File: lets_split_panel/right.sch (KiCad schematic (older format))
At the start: 69 parts, among them J4 RST, J5 Speaker, J6 ISP, P5 USB_OTG, P6 >WS2812, P7 WS2812>, P8 Conn_01x04, SW25 MXALPS, SW26 MXALPS, SW27 MXALPS, SW28 MXALPS, SW29 MXALPS, SW30 MXALPS, SW31 MXALPS, SW32 MXALPS, SW33 MXALPS, SW34 MXALPS, SW35 MXALPS, SW36 MXALPS, SW37 MXALPS, SW38 MXALPS, SW39 MXALPS, SW40 MXALPS, SW41 MXALPS, SW42 MXALPS, SW43 MXALPS, SW44 MXALPS, SW45 MXALPS, SW46 MXALPS, SW47 MXALPS, SW48 MXALPS, U2 ATMega32U4, Y2 Crystal

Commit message: Finished panel
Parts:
- removed JP3, JP4: I2C pullup, Jumpers:Solder-jumper-NO, symbol Jumper
- removed R11, R12: 4k7, Resistors_SMD:R_0603_HandSoldering, symbol R_Small
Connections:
- net labels added: Dd+, Dd-
- wire segments 132 -> 124
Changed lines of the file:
@@
 	1    0    0    -1
 $EndComp
-Text GLabel 4225 6625 2    55   Input ~ 0
+Text Label 4225 6625 0    55   ~ 0
 col0
-Text GLabel 4225 6725 2    55   Input ~ 0
+Text Label 4225 6725 0    55   ~ 0
 col1
-Text GLabel 4225 6275 2    55   Input ~ 0
+Text Label 4225 6275 0    55   ~ 0
 col2
-Text GLabel 4225 4925 2    55   Input ~ 0
+Text Label 4225 4925 0    55   ~ 0
 col3
-Text GLabel 4225 6125 2    55   Input ~ 0
+Text Label 4225 6125 0    55   ~ 0
 col4
-Text GLabel 4225 6025 2    55   Input ~ 0
+Text Label 4225 6025 0    55   ~ 0
 col5
-Text GLabel 4225 7025 2    55   Input ~ 0
+Text Label 4225 7025 0    55   ~ 0
 row3
-Text GLabel 4225 5275 2    55   Input ~ 0
+Text Label 4225 5275 0    55   ~ 0
 row2
-Text GLabel 4225 6925 2    55   Input ~ 0
+Text Label 4225 6925 0    55   ~ 0
 row1
-Text GLabel 4225 6825 2    55   Input ~ 0
+Text Label 4225 6825 0    55   ~ 0
 row0
 $Comp
@@
 	1    0    0    -1
 $EndComp
-$Comp
-L R_Small R12
-U 1 1 5A0E2942
-P 3525 1750
-F 0 "R12" H 3555 1770 50  0000 L CNN
-F 1 "4k7" H 3555 1710 50  0000 L CNN
-F 2 "Resistors_SMD:R_0603_HandSoldering" H 3525 1750 50  0001 C CNN
-F 3 "" H 3525 1750 50  0000 C CNN
-	1    3525 1750
-	1    0    0    -1
-$EndComp
-$Comp
-L R_Small R11
-U 1 1 5A0E2948
-P 3425 1750
-F 0 "R11" H 3455 1770 50  0000 L CNN
-F 1 "4k7" H 3455 1710 50  0000 L CNN
-F 2 "Resistors_SMD:R_0603_HandSoldering" H 3425 1750 50  0001 C CNN
-F 3 "" H 3425 1750 50  0000 C CNN
-	1    3425 1750
-	-1   0    0    -1
-$EndComp
-$Comp
-L Jumper JP3
-U 1 1 5A0E294E
-P 3425 1300
-F 0 "JP3" H 3425 1450 50  0000 C CNN
-F 1 "I2C pullup" H 3425 1525 50  0000 C CNN
-F 2 "Jumpers:Solder-jumper-NO" H 3425 1300 50  0001 C CNN
-F 3 "" H 3425 1300 50  0000 C CNN
-	1    3425 1300
-	0    -1   1    0
-$EndComp
-$Comp
-L VCC #PWR024
-U 1 1 5A0E2954
-P 3475 925
-F 0 "#PWR024" H 3475 775 50  0001 C CNN
-F 1 "VCC" H 3475 1075 50  0000 C CNN
-F 2 "" H 3475 925 50  0000 C CNN
-F 3 "" H 3475 925 50  0000 C CNN
-	1    3475 925
-	1    0    0    -1
-$EndComp
-Text GLabel 3675 1900 2    55   Output ~ 0
-SDA
-Text GLabel 3675 2000 2    55   Output ~ 0
+Text Label 7400 2900 2    55   ~ 0
 SCL/D3
-Text GLabel 7400 2900 0    55   Input ~ 0
-SCL/D3
-Text GLabel 7400 2800 0    55   Input ~ 0
+Text Label 7400 2800 2    55   ~ 0
 SDA
 $Comp
 L USB_OTG-RESCUE-lets_split P5
 U 1 1 5A0E295E
-P 1225 5525
-F 0 "P5" H 1550 5400 50  0000 C CNN
-F 1 "USB_OTG" H 1225 5725 50  0000 C CNN
-F 2 "Connectors:USB-Mini-B-SMD" V 1175 5425 50  0001 C CNN
-F 3 "" V 1175 5425 50  0000 C CNN
-	1    1225 5525
+P 1150 5525
+F 0 "P5" H 1475 5400 50  0000 C CNN
+F 1 "USB_OTG" H 1150 5725 50  0000 C CNN
+F 2 "Connectors:USB-Mini-B-SMD" V 1100 5425 50  0001 C CNN
+F 3 "" V 1100 5425 50  0000 C CNN
+	1    1150 5525
 	0    -1   1    0
 $EndComp
@@
 	1    0    0    -1
 $EndComp
-Text GLabel 4250 6525 2    55   Output ~ 0
+Text Label 4250 6525 0    55   ~ 0
 WD2812-in
-Text GLabel 3075 2525 0    55   Input ~ 0
+Text Label 3075 2525 2    55   ~ 0
 WD2812-in
 $Comp
@@
 	-1   0    0    -1
 $EndComp
-Text GLabel 3900 2525 2    55   Output ~ 0
+Text Label 3900 2525 0    55   ~ 0
 SDA
-Text GLabel 3275 1900 0    55   Input ~ 0
+Text Label 4275 5525 0    55   ~ 0
 SDA
-Text GLabel 3275 2000 0    55   Input ~ 0
+Text Label 4275 5425 0    55   ~ 0
 SCL/D3
-Text GLabel 4275 5525 2    55   Output ~ 0
-SDA
-Text GLabel 4275 5425 2    55   Output ~ 0
-SCL/D3
-Text GLabel 4275 5175 2    60   Output ~ 0
+Text Label 4275 5175 0    60   ~ 0
 buzz
-Text GLabel 3200 3125 0    60   Input ~ 0
+Text Label 3200 3125 2    60   ~ 0
 buzz
 $Comp
@@
 L VBUS #PWR031
 U 1 1 5A0E29DF
-P 1575 5275
-F 0 "#PWR031" H 1575 5125 50  0001 C CNN
-F 1 "VBUS" H 1590 5448 50  0000 C CNN
-F 2 "" H 1575 5275 50  0001 C CNN
-F 3 "" H 1575 5275 50  0001 C CNN
-	1    1575 5275
+P 1500 5275
+F 0 "#PWR031" H 1500 5125 50  0001 C CNN
+F 1 "VBUS" H 1515 5448 50  0000 C CNN
+F 2 "" H 1500 5275 50  0001 C CNN
+F 3 "" H 1500 5275 50  0001 C CNN
+	1    1500 5275
 	1    0    0    -1
 $EndComp
@@
 L GND #PWR033
 U 1 1 5A0E29EB
-P 1125 6050
-F 0 "#PWR033" H 1125 5800 50  0001 C CNN
-F 1 "GND" H 1125 5900 50  0000 C CNN
-F 2 "" H 1125 6050 50  0000 C CNN
-F 3 "" H 1125 6050 50  0000 C CNN
-	1    1125 6050
+P 1050 6050
+F 0 "#PWR033" H 1050 5800 50  0001 C CNN
+F 1 "GND" H 1050 5900 50  0000 C CNN
+F 2 "" H 1050 6050 50  0000 C CNN
+F 3 "" H 1050 6050 50  0000 C CNN
+	1    1050 6050
 	1    0    0    -1
 $EndComp
@@
 	2350 4200 2350 5225
 Wire Wire Line
-	3275 2000 3675 2000
-Wire Wire Line
-	3525 2000 3525 1850
-Wire Wire Line
-	3275 1900 3675 1900
-Wire Wire Line
-	3425 1900 3425 1850
-Wire Wire Line
-	3425 1650 3425 1600
-Wire Wire Line
-	3525 1600 3525 1650
-Connection ~ 3425 1900
-Connection ~ 3525 2000
-Wire Wire Line
 	7350 3150 7350 3100
 Wire Wire Line
@@
 	2625 5525 1725 5525
 Wire Wire Line
-	1525 5325 1575 5325
-Wire Wire Line
-	1575 5325 1575 5275
-Wire Wire Line
-	1125 5925 1125 6050
+	1450 5325 1500 5325
+Wire Wire Line
+	1500 5325 1500 5275
+Wire Wire Line
+	1050 5925 1050 6050
 Wire Wire Line
 	2100 5725 2275 5725
@@
 	2100 5725 2100 6200
 Wire Wire Line
-	1125 5975 1575 5975
-Wire Wire Line
-	1575 5975 1575 5725
-Wire Wire Line
-	1575 5725 1525 5725
-Connection ~ 1125 5975
+	1050 5975 1500 5975
+Wire Wire Line
+	1500 5975 1500 5725
+Wire Wire Line
+	1500 5725 1450 5725
+Connection ~ 1050 5975
 $Comp
 L VBUS #PWR034
@@
 	4225 6525 4250 6525
 $Comp
-L Jumper JP4
-U 1 1 5A0E2A65
-P 3525 1300
-F 0 "JP4" H 3525 1450 50  0000 C CNN
-F 1 "I2C pullup" H 3525 1525 50  0000 C CNN
-F 2 "Jumpers:Solder-jumper-NO" H 3525 1300 50  0001 C CNN
-F 3 "" H 3525 1300 50  0000 C CNN
-	1    3525 1300
-	0    1    1    0
-$EndComp
-Wire Wire Line
-	3425 1000 3425 975
-Wire Wire Line
-	3425 975  3525 975
-Wire Wire Line
-	3525 975  3525 1000
-Wire Wire Line
-	3475 975  3475 925
-Connection ~ 3475 975
-$Comp
 L Conn_02x03_Odd_Even J6
 U 1 1 5A0E2A70
@@
 	1    0    0    -1
 $EndComp
-Text GLabel 5575 6800 0    35   Output ~ 0
+Text Label 5575 6800 2    55   ~ 0
 ~RESET
-Text GLabel 5575 6600 0    55   Input ~ 0
-MISO
-Text GLabel 5575 6700 0    55   Output ~ 0
+Text Label 5575 6700 2    55   ~ 0
 SCK
-Text GLabel 6075 6700 2    55   Output ~ 0
-MOSI
-Text GLabel 1925 4725 1    35   Input ~ 0
+Text Label 1925 4725 1    35   ~ 0
 ~RESET
 Wire Wire Line
 	1925 4725 1925 4775
 Connection ~ 1925 4775
-Text GLabel 4225 4525 2    55   Input ~ 0
+Text Label 4225 4525 0    55   ~ 0
 MOSI
-Text GLabel 4225 4625 2    55   Output ~ 0
+Text Label 4225 4625 0    55   ~ 0
 MISO
-Text GLabel 4225 4425 2    55   Input ~ 0
+Text Label 4225 4425 0    55   ~ 0
 SCK
 Wire Wire Line
@@
 $EndComp
 Wire Wire Line
-	10000 4825 9875 4825
+	9875 4825 10000 4825
 Wire Wire Line
 	10400 4825 10475 4825
@@
 $EndComp
 Wire Wire Line
-	9250 4825 9125 4825
+	9125 4825 9250 4825
 Wire Wire Line
 	9650 4825 9725 4825
@@
 $EndComp
 Wire Wire Line
-	8500 4825 8375 4825
+	8375 4825 8500 4825
 Wire Wire Line
 	8900 4825 8975 4825
@@
 $EndComp
 Wire Wire Line
-	7750 4825 7625 4825
+	7625 4825 7750 4825
 Wire Wire Line
 	8150 4825 8225 4825
@@
 $EndComp
 Wire Wire Line
-	7050 4825 6925 4825
+	6925 4825 7050 4825
 Wire Wire Line
 	7450 4825 7525 4825
@@
 $EndComp
 Wire Wire Line
-	6300 4825 6175 4825
+	6175 4825 6300 4825
 Wire Wire Line
 	6700 4825 6775 4825
@@
 $EndComp
 Wire Wire Line
-	10000 4325 9875 4325
+	9875 4325 10000 4325
 Wire Wire Line
 	10400 4325 10475 4325
@@
 $EndComp
 Wire Wire Line
-	9250 4325 9125 4325
+	9125 4325 9250 4325
 Wire Wire Line
 	9650 4325 9725 4325
@@
 $EndComp
 Wire Wire Line
-	8500 4325 8375 4325
+	8375 4325 8500 4325
 Wire Wire Line
 	8900 4325 8975 4325
@@
 $EndComp
 Wire Wire Line
-	7750 4325 7625 4325
+	7625 4325 7750 4325
 Wire Wire Line
 	8150 4325 8225 4325
@@
 $EndComp
 Wire Wire Line
-	7050 4325 6925 4325
+	6925 4325 7050 4325
 Wire Wire Line
 	7450 4325 7525 4325
@@
 $EndComp
 Wire Wire Line
-	6300 4325 6175 4325
+	6175 4325 6300 4325
 Wire Wire Line
 	6700 4325 6775 4325
@@
 Wire Wire Line
 	6775 4125 10475 4125
-Text GLabel 6775 5625 0    60   Input ~ 0
+Text Label 6775 5625 2    60   ~ 0
 row3
-Text GLabel 6775 5125 0    60   Input ~ 0
+Text Label 6775 5125 2    60   ~ 0
 row2
-Text GLabel 6775 4625 0    60   Input ~ 0
+Text Label 6775 4625 2    60   ~ 0
 row1
-Text GLabel 6775 4125 0    60   Input ~ 0
+Text Label 6775 4125 2    60   ~ 0
 row0
-Text GLabel 9875 3775 1    60   Input ~ 0
+Text Label 9875 3775 1    60   ~ 0
 col5
-Text GLabel 9125 3775 1    60   Input ~ 0
+Text Label 9125 3775 1    60   ~ 0
 col4
-Text GLabel 8375 3775 1    60   Input ~ 0
+Text Label 8375 3775 1    60   ~ 0
 col3
-Text GLabel 7625 3775 1    60   Input ~ 0
+Text Label 7625 3775 1    60   ~ 0
 col2
-Text GLabel 6925 3775 1    60   Input ~ 0
+Text Label 6925 3775 1    60   ~ 0
 col1
-Text GLabel 6175 3775 1    60   Input ~ 0
+Text Label 6175 3775 1    60   ~ 0
 col0
 $Comp
@@
 	0    -1   -1   0
 $EndComp
+Text Label 5575 6600 2    55   ~ 0
+MISO
+Text Label 6075 6700 0    55   ~ 0
+MOSI
+Text Label 1450 5425 0    60   ~ 0
+Dd-
+Wire Wire Line
+	1450 5425 1525 5425
+Text Label 1450 5525 0    60   ~ 0
+Dd+
+Wire Wire Line
+	1450 5525 1525 5525
 $EndSCHEMATC

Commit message: Added test jig for panel
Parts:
- removed P7: WS2812>, Wirepads:SMD_PAD_1x03_Pitch2.54mm, symbol Conn_01x03
- added J8: WS2812>, Pin_Headers:Pin_Header_Straight_1x01_Pitch2.54mm, symbol conn:Conn_01x01
- C5, C6, C7, C8: symbol C_Small -> lets_split_panel-rescue:C_Small-RESCUE-lets_split_panel
- D25, D26, D27, D28, D29, D30, D31, D32, D33, D34, D35, D36, D37, D38, D39, D40, D41, D42, D43, D44, D45, D46, D47, D48: symbol D -> lets_split_panel-rescue:D-RESCUE-lets_split_panel
- J4, J5: symbol Conn_01x02 -> lets_split_panel-rescue:Conn_01x02-RESCUE-lets_split_panel
- J6: footprint Jlink:J-link-needle-6pin -> Pin_Headers:Pin_Header_Straight_2x03_Pitch2.54mm; symbol Conn_02x03_Odd_Even -> lets_split_panel-rescue:Conn_02x03_Odd_Even-RESCUE-lets_split_panel
- P5: symbol USB_OTG-RESCUE-lets_split -> lets_split_panel-rescue:USB_OTG-RESCUE-lets_split-RESCUE-lets_split_panel
- P6: symbol Conn_01x03 -> lets_split_panel-rescue:Conn_01x03-RESCUE-lets_split_panel
- P8: symbol Conn_01x04 -> lets_split_panel-rescue:Conn_01x04-RESCUE-lets_split_panel
- R10, R7, R8, R9: symbol R_Small -> lets_split_panel-rescue:R_Small-RESCUE-lets_split_panel
- SW25, SW26, SW27, SW28, SW29, SW30, SW31, SW32, SW33, SW34, SW35, SW36, SW37, SW38, SW39, SW40, SW41, SW42, SW43, SW44, SW45, SW46, SW47, SW48: symbol MXALPS -> lets_split_panel-rescue:MXALPS-RESCUE-lets_split_panel
- U2: symbol ATMega32U4 -> lets_split_panel-rescue:ATMega32U4-RESCUE-lets_split_panel
- Y2: symbol Crystal -> lets_split_panel-rescue:Crystal-RESCUE-lets_split_panel
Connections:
- wire segments 124 -> 120

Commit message: Changed to use SOT-23 dual diodes for cost
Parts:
- removed D25, D26, D27, D28, D29, D30, D31, D32, D33, D34, D35, D36, D37, D38, D39, D40, D41, D42, D43, D44, D45, D46, D47, D48: D, SeeedOPL-Diode-2016:SOD-123, symbol lets_split_panel-rescue:D-RESCUE-lets_split_panel
- removed SW25, SW26, SW27, SW28, SW29, SW30, SW31, SW32, SW33, SW34, SW35, SW36, SW37, SW38, SW39, SW40, SW41, SW42, SW43, SW44, SW45, SW46, SW47, SW48: MXALPS, CherryMX:Kailh-socket, symbol lets_split_panel-rescue:MXALPS-RESCUE-lets_split_panel
- added D13, D14, D15, D16, D17, D18, D19, D20, D21, D22, D23, D24: D_x2_KCom_AAK, TO_SOT_Packages_SMD:SOT-23, symbol device:D_x2_KCom_AAK
- added SW25, SW26, SW27, SW28, SW29, SW30, SW31, SW32, SW33, SW34, SW35, SW36, SW37, SW38, SW39, SW40, SW41, SW42, SW43, SW44, SW45, SW46, SW47, SW48: Socket, CherryMX:Kailh-socket, symbol switches:SW_Push
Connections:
- wire segments 120 -> 108
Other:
- moved on the sheet: P8

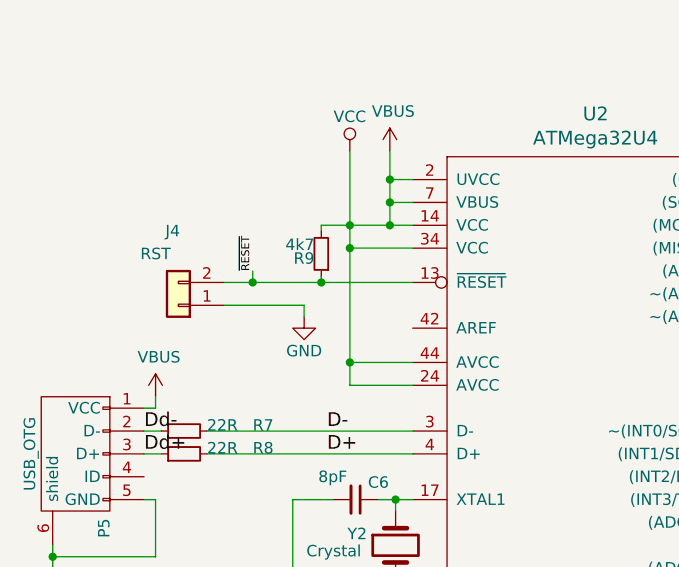
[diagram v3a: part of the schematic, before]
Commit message: Added fancy :)
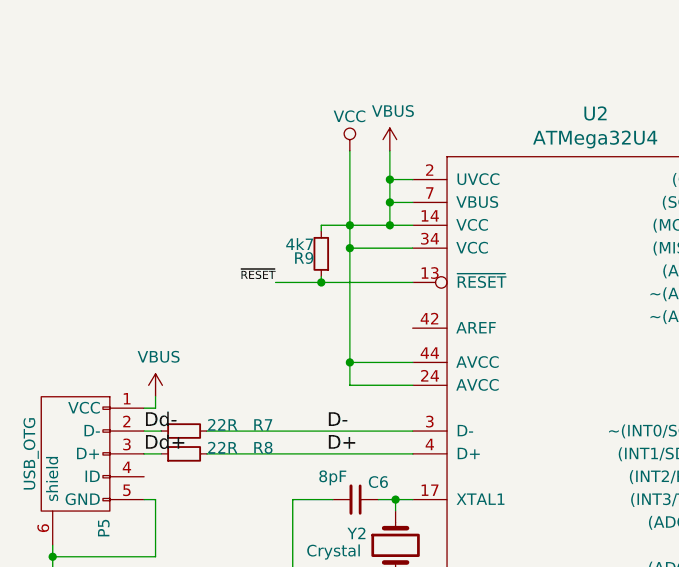
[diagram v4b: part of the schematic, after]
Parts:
- removed J4: RST, Pin_Headers:Pin_Header_Straight_1x02_Pitch2.54mm, symbol lets_split_panel-rescue:Conn_01x02-RESCUE-lets_split_panel
- C5, C8: footprint SeeedOPL-Capacitor-2016:C0603 -> Capacitors_SMD:C_0603
- C6, C7: footprint SeeedOPL-Capacitor-2016:C0402 -> Capacitors_SMD:C_0603
- R10, R7, R8, R9: footprint Resistors_SMD:R_0603_HandSoldering -> Resistors_SMD:R_0603
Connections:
- wire segments 108 -> 105
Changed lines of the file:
@@
 F 0 "R10" H 3330 3145 50  0000 L CNN
 F 1 "200" H 3330 3085 50  0000 L CNN
-F 2 "Resistors_SMD:R_0603_HandSoldering" H 3300 3125 50  0001 C CNN
+F 2 "Resistors_SMD:R_0603" H 3300 3125 50  0001 C CNN
 F 3 "" H 3300 3125 50  0000 C CNN
 	1    3300 3125
@@
 F 0 "R9" H 2255 4670 50  0000 L CNN
 F 1 "4k7" H 2255 4610 50  0000 L CNN
-F 2 "Resistors_SMD:R_0603_HandSoldering" H 2225 4650 50  0001 C CNN
+F 2 "Resistors_SMD:R_0603" H 2225 4650 50  0001 C CNN
 F 3 "" H 2225 4650 50  0000 C CNN
 	1    2225 4650
@@
 F 0 "C8" H 2567 6521 50  0000 L CNN
 F 1 "1uF" H 2567 6430 50  0000 L CNN
-F 2 "SeeedOPL-Capacitor-2016:C0603" H 2475 6475 50  0001 C CNN
+F 2 "Capacitors_SMD:C_0603" H 2475 6475 50  0001 C CNN
 F 3 "" H 2475 6475 50  0001 C CNN
 	1    2475 6475
@@
 F 0 "C6" V 2300 5825 50  0000 C CNN
 F 1 "8pF" V 2275 5625 50  0000 C CNN
-F 2 "SeeedOPL-Capacitor-2016:C0402" H 2375 5725 50  0001 C CNN
+F 2 "Capacitors_SMD:C_0603" H 2375 5725 50  0001 C CNN
 F 3 "" H 2375 5725 50  0001 C CNN
 	1    2375 5725
@@
 F 0 "C7" V 2550 6125 50  0000 C CNN
 F 1 "8pF" V 2475 6125 50  0000 C CNN
-F 2 "SeeedOPL-Capacitor-2016:C0402" H 2375 6125 50  0001 C CNN
+F 2 "Capacitors_SMD:C_0603" H 2375 6125 50  0001 C CNN
 F 3 "" H 2375 6125 50  0001 C CNN
 	1    2375 6125
@@
 F 0 "R7" V 1650 5125 50  0000 R CNN
 F 1 "22R" V 1650 5325 50  0000 R CNN
-F 2 "Resistors_SMD:R_0603_HandSoldering" H 1625 5425 50  0001 C CNN
+F 2 "Resistors_SMD:R_0603" H 1625 5425 50  0001 C CNN
 F 3 "" H 1625 5425 50  0000 C CNN
 	1    1625 5425
@@
 F 0 "R8" V 1650 5225 50  0000 R CNN
 F 1 "22R" V 1650 5425 50  0000 R CNN
-F 2 "Resistors_SMD:R_0603_HandSoldering" H 1625 5525 50  0001 C CNN
+F 2 "Resistors_SMD:R_0603" H 1625 5525 50  0001 C CNN
 F 3 "" H 1625 5525 50  0000 C CNN
 	1    1625 5525
@@
 F 0 "C5" H 2267 7071 50  0000 L CNN
 F 1 "1uF" H 2267 6980 50  0000 L CNN
-F 2 "SeeedOPL-Capacitor-2016:C0603" H 2175 7025 50  0001 C CNN
+F 2 "Capacitors_SMD:C_0603" H 2175 7025 50  0001 C CNN
 F 3 "" H 2175 7025 50  0001 C CNN
 	1    2175 7025
@@
 Wire Wire Line
 	2225 4775 2225 4750
-Wire Wire Line
-	1800 4775 2625 4775
 Connection ~ 2225 4775
 Wire Wire Line
@@
 	-1   0    0    -1
 $EndComp
-$Comp
-L lets_split_panel-rescue:Conn_01x02-RESCUE-lets_split_panel J4
-U 1 1 5A0E2A4F
-P 1600 4875
-F 0 "J4" H 1625 4550 50  0000 C CNN
-F 1 "RST" H 1700 4650 50  0000 C CNN
-F 2 "Pin_Headers:Pin_Header_Straight_1x02_Pitch2.54mm" H 1600 4875 50  0001 C CNN
-F 3 "" H 1600 4875 50  0001 C CNN
-	1    1600 4875
-	-1   0    0    1
-$EndComp
-$Comp
-L lets_split_panel-rescue:GND-RESCUE-lets_split_panel #PWR036
-U 1 1 5A0E2A55
-P 2150 4925
-F 0 "#PWR036" H 2150 4675 50  0001 C CNN
-F 1 "GND" H 2150 4775 50  0000 C CNN
-F 2 "" H 2150 4925 50  0000 C CNN
-F 3 "" H 2150 4925 50  0000 C CNN
-	1    2150 4925
-	1    0    0    -1
-$EndComp
-Wire Wire Line
-	1800 4875 2150 4875
-Wire Wire Line
-	2150 4875 2150 4925
 Wire Wire Line
 	2625 6525 2575 6525
@@
 Text Label 5575 6700 2    55   ~ 0
 SCK
-Text Label 1925 4725 1    35   ~ 0
+Text Label 2025 4775 2    35   ~ 0
 ~RESET
-Wire Wire Line
-	1925 4725 1925 4775
-Connection ~ 1925 4775
 Text Label 4225 4525 0    55   ~ 0
 MOSI
@@
 Connection ~ 10700 3875
 Connection ~ 10700 3225
+Wire Wire Line
+	2025 4775 2625 4775
 $EndSCHEMATC

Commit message: Seperated gerbers on request from board house
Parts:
- J8: symbol conn:Conn_01x01 -> lets_split_panel-rescue:Conn_01x01-RESCUE-lets_split_panel
- SW25, SW26, SW27, SW28, SW29, SW30, SW31, SW32, SW33, SW34, SW35, SW36, SW37, SW38, SW39, SW40, SW41, SW42, SW43, SW44, SW45, SW46, SW47, SW48: symbol switches:SW_Push -> lets_split_panel-rescue:SW_Push-RESCUE-lets_split_panel
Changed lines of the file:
@@
 	1450 5525 1525 5525
 $Comp
-L conn:Conn_01x01 J8
+L lets_split_panel-rescue:Conn_01x01-RESCUE-lets_split_panel J8
 U 1 1 5A14BD9C
 P 3675 2525
@@
 $EndComp
 $Comp
-L switches:SW_Push SW25
+L lets_split_panel-rescue:SW_Push-RESCUE-lets_split_panel SW25
 U 1 1 5A17DCD0
 P 6250 3225
@@
 Connection ~ 8350 3475
 $Comp
-L switches:SW_Push SW26
+L lets_split_panel-rescue:SW_Push-RESCUE-lets_split_panel SW26
 U 1 1 5A17DCF7
 P 7250 3225
@@
 $EndComp
 $Comp
-L switches:SW_Push SW27
+L lets_split_panel-rescue:SW_Push-RESCUE-lets_split_panel SW27
 U 1 1 5A17DCFE
 P 7850 3225
@@
 $EndComp
 $Comp
-L switches:SW_Push SW28
+L lets_split_panel-rescue:SW_Push-RESCUE-lets_split_panel SW28
 U 1 1 5A17DD05
 P 8850 3225
@@
 $EndComp
 $Comp
-L switches:SW_Push SW29
+L lets_split_panel-rescue:SW_Push-RESCUE-lets_split_panel SW29
 U 1 1 5A17DD0C
 P 9450 3225
@@
 $EndComp
 $Comp
-L switches:SW_Push SW30
+L lets_split_panel-rescue:SW_Push-RESCUE-lets_split_panel SW30
 U 1 1 5A17DD13
 P 10450 3225
@@
 $EndComp
 $Comp
-L switches:SW_Push SW31
+L lets_split_panel-rescue:SW_Push-RESCUE-lets_split_panel SW31
 U 1 1 5A17DD21
 P 6250 3875
@@
 Connection ~ 8350 4125
 $Comp
-L switches:SW_Push SW32
+L lets_split_panel-rescue:SW_Push-RESCUE-lets_split_panel SW32
 U 1 1 5A17DD42
 P 7250 3875
@@
 $EndComp
 $Comp
-L switches:SW_Push SW33
+L lets_split_panel-rescue:SW_Push-RESCUE-lets_split_panel SW33
 U 1 1 5A17DD49
 P 7850 3875
@@
 $EndComp
 $Comp
-L switches:SW_Push SW34
+L lets_split_panel-rescue:SW_Push-RESCUE-lets_split_panel SW34
 U 1 1 5A17DD50
 P 8850 3875
@@
 $EndComp
 $Comp
-L switches:SW_Push SW35
+L lets_split_panel-rescue:SW_Push-RESCUE-lets_split_panel SW35
 U 1 1 5A17DD57
 P 9450 3875
@@
 $EndComp
 $Comp
-L switches:SW_Push SW36
+L lets_split_panel-rescue:SW_Push-RESCUE-lets_split_panel SW36
 U 1 1 5A17DD5E
 P 10450 3875
@@
 $EndComp
 $Comp
-L switches:SW_Push SW37
+L lets_split_panel-rescue:SW_Push-RESCUE-lets_split_panel SW37
 U 1 1 5A17DD6C
 P 6250 4525
@@
 Connection ~ 8350 4775
 $Comp
-L switches:SW_Push SW38
+L lets_split_panel-rescue:SW_Push-RESCUE-lets_split_panel SW38
 U 1 1 5A17DD8D
 P 7250 4525
@@
 $EndComp
 $Comp
-L switches:SW_Push SW39
+L lets_split_panel-rescue:SW_Push-RESCUE-lets_split_panel SW39
 U 1 1 5A17DD94
 P 7850 4525
@@
 $EndComp
 $Comp
-L switches:SW_Push SW40
+L lets_split_panel-rescue:SW_Push-RESCUE-lets_split_panel SW40
 U 1 1 5A17DD9B
 P 8850 4525
@@
 $EndComp
 $Comp
-L switches:SW_Push SW41
+L lets_split_panel-rescue:SW_Push-RESCUE-lets_split_panel SW41
 U 1 1 5A17DDA2
 P 9450 4525
@@
 $EndComp
 $Comp
-L switches:SW_Push SW42
+L lets_split_panel-rescue:SW_Push-RESCUE-lets_split_panel SW42
 U 1 1 5A17DDA9
 P 10450 4525
@@
 $EndComp
 $Comp
-L switches:SW_Push SW43
+L lets_split_panel-rescue:SW_Push-RESCUE-lets_split_panel SW43
 U 1 1 5A17DDB7
 P 6250 5175
@@
 Connection ~ 8350 5425
 $Comp
-L switches:SW_Push SW44
+L lets_split_panel-rescue:SW_Push-RESCUE-lets_split_panel SW44
 U 1 1 5A17DDD8
 P 7250 5175
@@
 $EndComp
 $Comp
-L switches:SW_Push SW45
+L lets_split_panel-rescue:SW_Push-RESCUE-lets_split_panel SW45
 U 1 1 5A17DDDF
 P 7850 5175
@@
 $EndComp
 $Comp
-L switches:SW_Push SW46
+L lets_split_panel-rescue:SW_Push-RESCUE-lets_split_panel SW46
 U 1 1 5A17DDE6
 P 8850 5175
@@
 $EndComp
 $Comp
-L switches:SW_Push SW47
+L lets_split_panel-rescue:SW_Push-RESCUE-lets_split_panel SW47
 U 1 1 5A17DDED
 P 9450 5175
@@
 $EndComp
 $Comp
-L switches:SW_Push SW48
+L lets_split_panel-rescue:SW_Push-RESCUE-lets_split_panel SW48
 U 1 1 5A17DDF4
 P 10450 5175
